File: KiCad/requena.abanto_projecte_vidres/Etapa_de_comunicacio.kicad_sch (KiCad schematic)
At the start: 5 parts, among them J1 DE9_Pins, J2 DE9_Pins, U1 CP2102N-Axx-xQFN20, U2 MAX3232, U3 TJA1051TK-3

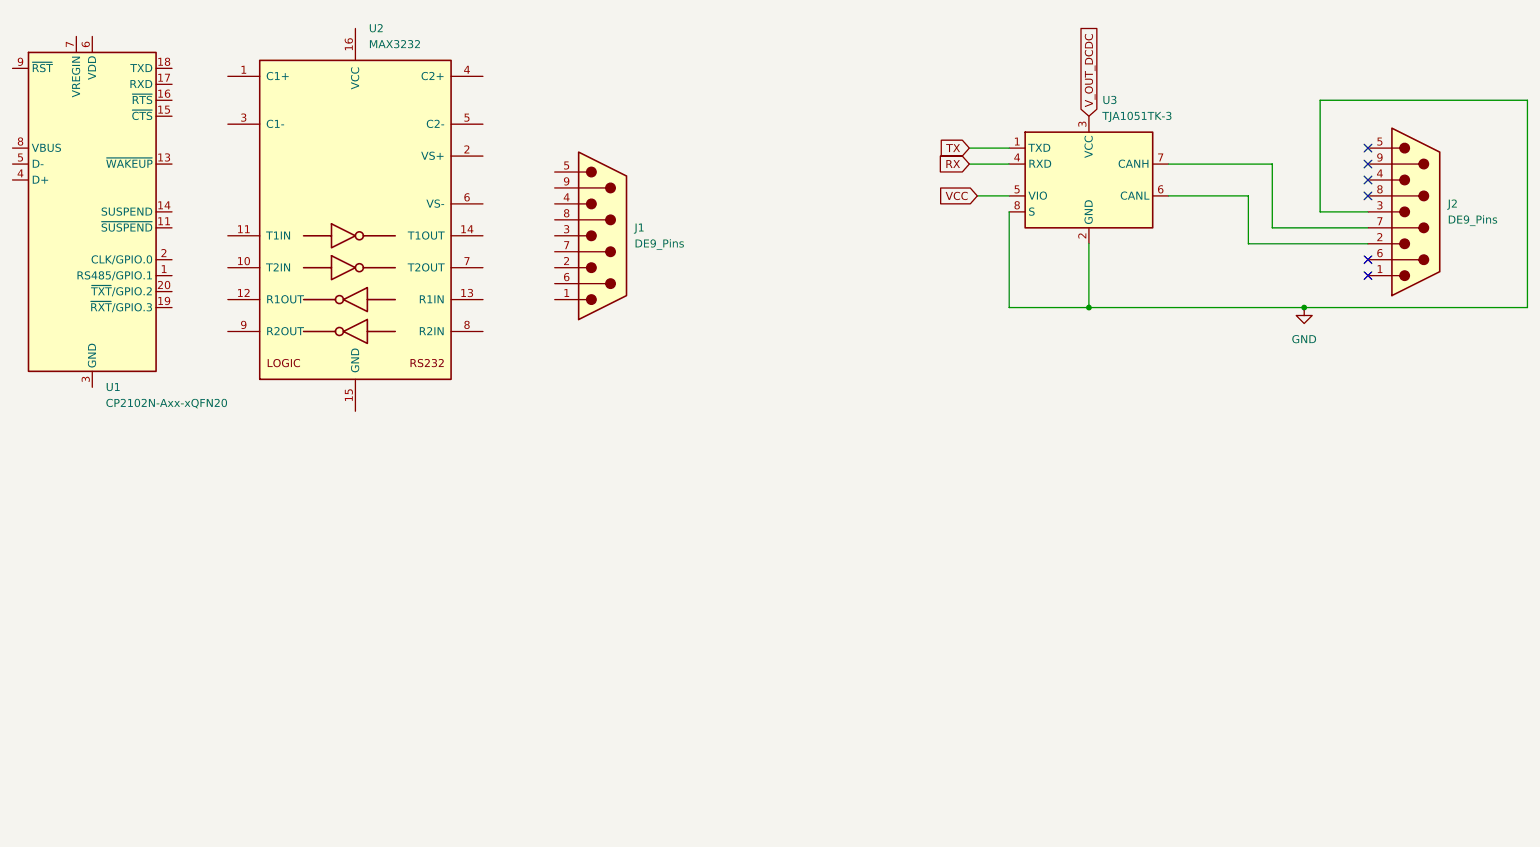
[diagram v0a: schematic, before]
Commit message: avance comunicaciones
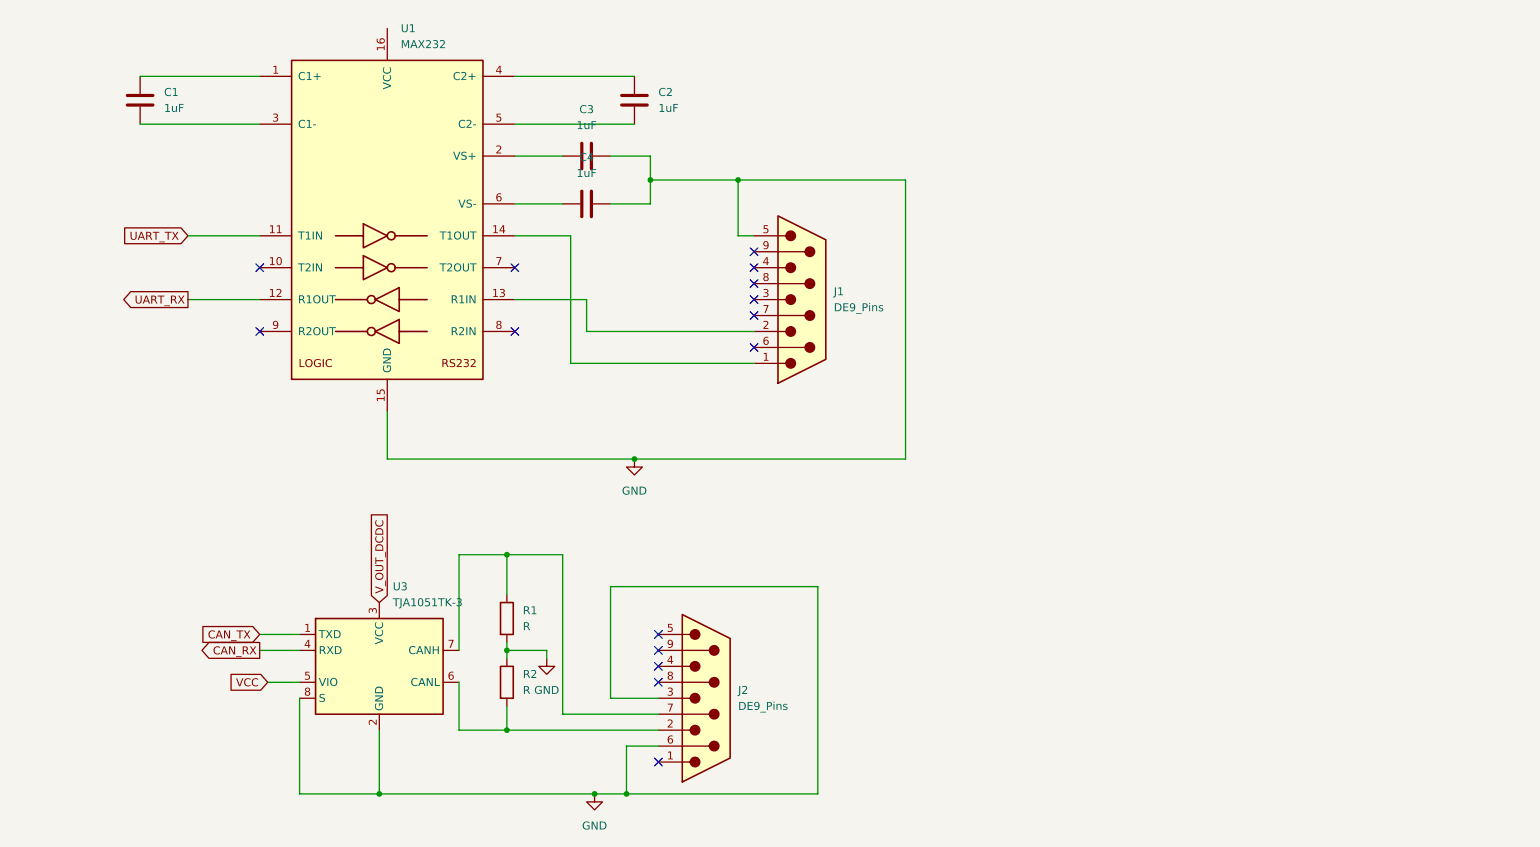
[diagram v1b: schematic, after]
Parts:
- removed U1: CP2102N-Axx-xQFN20, Package_DFN_QFN:SiliconLabs_QFN-20-1EP_3x3mm_P0.5mm, symbol Interface_USB:CP2102N-Axx-xQFN20
- removed U2: MAX3232, symbol Interface_UART:MAX3232
- added C1, C2, C3, C4: 1uF, symbol Device:C
- added R1, R2: R, symbol Device:R
- added U1: MAX232, symbol Interface_UART:MAX232
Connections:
- net GND: now also J1.5, J2.6, C3.2, C4.2, R1.2, R2.1, U1.15 (GND)
- net at J2.2, U3.6 (CANL): now also R2.2
- net at J2.7, U3.7 (CANH): now also R1.1
- net at J1.1: now also U1.14 (T1OUT)
- net at J1.2: now also U1.13 (R1IN)
- net RX renamed CAN_RX
- net TX renamed CAN_TX
- new net: C3.1, U1.2 (VS+)
- new net: C2.1, U1.4 (C2+)
- new net: C2.2, U1.5 (C2-)
- new net: C1.1, U1.1 (C1+)
- new net: C1.2, U1.3 (C1-)
- new net: C4.1, U1.6 (VS-)
- new net UART_RX: U1.12 (R1OUT)
- new net UART_TX: U1.11 (T1IN)
- no-connect marks 6 -> 15
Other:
- moved on the sheet: J1, J2, U3
